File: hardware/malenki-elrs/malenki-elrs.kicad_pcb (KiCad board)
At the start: 4 copper layers, 19 x 32 mm, 68 parts, among them J1 Conn_01x02_Male-Connector, J2 PROG Header, J3 Weapons, J4 Conn_01x02_Male-Connector, J5 Conn_01x02_Male-Connector, J6 Conn_01x02_Male-Connector, U1 SPX3819M5-L-3-3, U2 ESP32-S3FN8, U3 SX1280IMLTRT, U4 DRV8837DSGR, U5 DRV8837DSGR, U6 DRV8837DSGR, Y1 ECS-400-10-37B2-CKY-TR, Y2 CRYSTAL 52MHz 10pF SMD

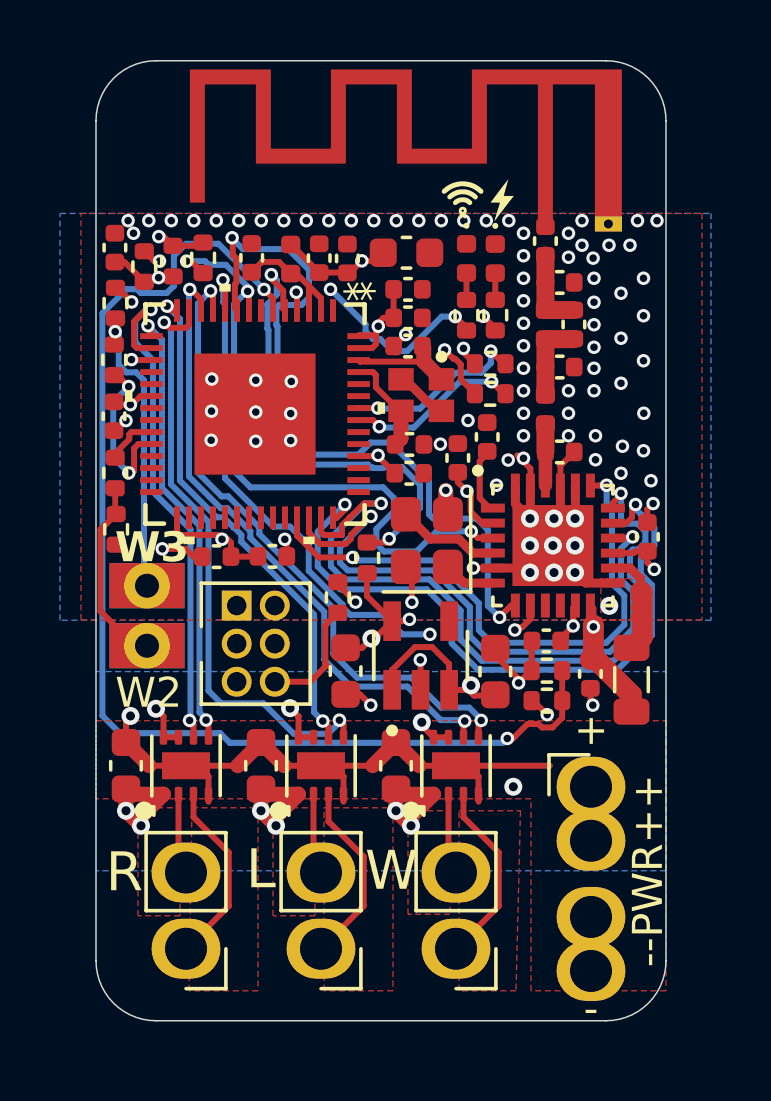
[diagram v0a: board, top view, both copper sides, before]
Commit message: added application note for antenna and final updated production files.
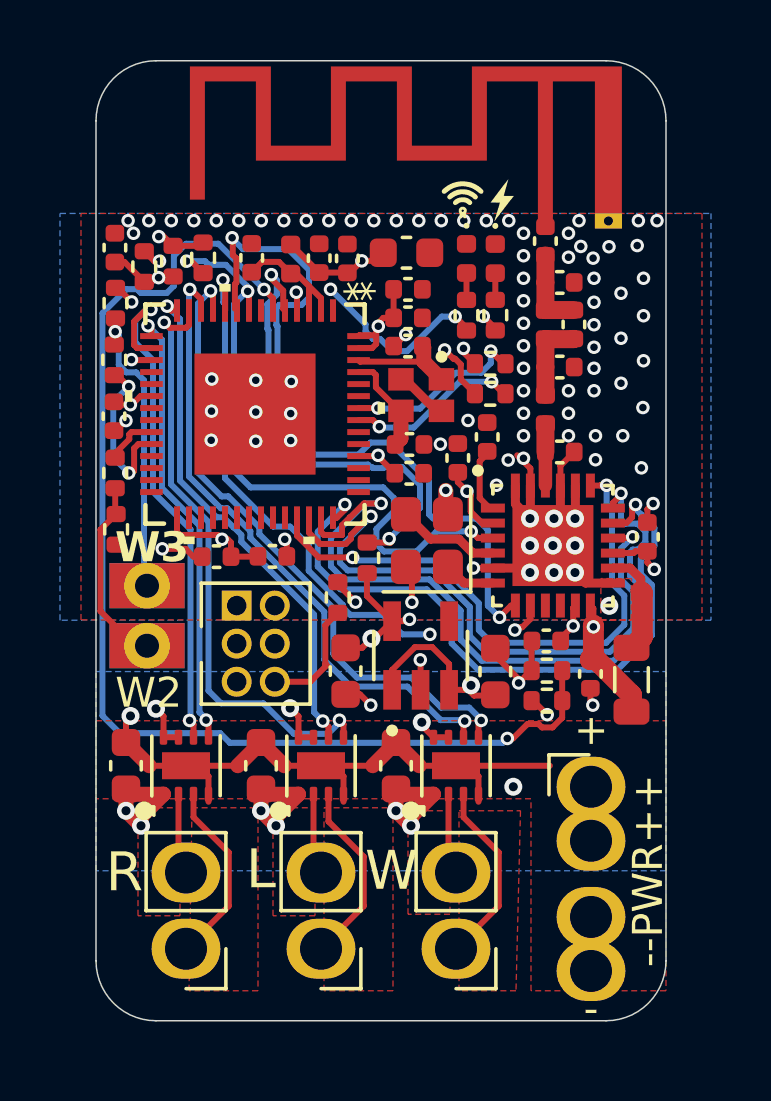
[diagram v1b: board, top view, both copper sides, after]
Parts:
- G***: moved to B.Cu
- moved G*** 9.28 mm to (97.3, 56.9), turned to 180 degrees
- moved AE1 0.10 mm to (103.0, 54.8)
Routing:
- net GND: vias 99 -> 97
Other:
- board text added: "Malenki-Nano Integrated Receiver"
- board text removed: "Malenki-Nano Integrated ExpressLRS Receiver"
